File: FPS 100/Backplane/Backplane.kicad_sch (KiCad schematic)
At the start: 27 parts

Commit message: 2026/1/7
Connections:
- net FAOVFL* is gone; now on net FAOVF*: 4401_FA_J1.32
- net FAUNFL* is gone; now on net FAUNF*: 4401_FA_J1.30
- net FAZERO* is gone; now on net FAZRO*: 4422_P1_J3.16
- net SCN is gone; now on net SCIN: 4401_FA_J1.33
- net DE07*: now also 4401_FA_J1.35; no longer 4401_FA_J1.37
- net FRCINH*: now reaches 4401_FA_J2.100
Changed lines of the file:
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@@
 		)
 	)
-	(global_label "FAUNFL*"
+	(global_label "FAUNF*"
 		(shape input)
 		(at 99.06 97.79 0)
@@
 		)
 		(property "Intersheetrefs" "${INTERSHEET_REFS}"
-			(at 109.9677 97.79 0)
+			(at 108.9396 97.79 0)
 			(effects
 				(font
@@
 	(global_label "DE07*"
 		(shape input)
-		(at 86.36 107.95 180)
+		(at 86.36 105.41 180)
 		(fields_autoplaced yes)
 		(effects
@@
 		)
 		(property "Intersheetrefs" "${INTERSHEET_REFS}"
-			(at 77.5692 107.95 0)
+			(at 77.5692 105.41 0)
 			(effects
 				(font
@@
 		)
 	)
-	(global_label "FAZERO*"
+	(global_label "FAZRO*"
 		(shape input)
 		(at 643.89 80.01 0)
@@
 		)
 		(property "Intersheetrefs" "${INTERSHEET_REFS}"
-			(at 654.979 80.01 0)
+			(at 653.83 80.01 0)
 			(effects
 				(font
@@
 		)
 	)
-	(global_label "FAOVFL*"
+	(global_label "FAOVF*"
 		(shape input)
 		(at 99.06 100.33 0)
@@
 		)
 		(property "Intersheetrefs" "${INTERSHEET_REFS}"
-			(at 109.7258 100.33 0)
+			(at 108.6977 100.33 0)
 			(effects
 				(font
@@
 		)
 	)
+	(global_label "FRCINH*"
+		(shape input)
+		(at 99.06 346.71 0)
+		(fields_autoplaced yes)
+		(effects
+			(font
+				(size 1.27 1.27)
+			)
+			(justify left)
+		)
+		(property "Intersheetrefs" "${INTERSHEET_REFS}"
+			(at 109.9072 346.71 0)
+			(effects
+				(font
+					(size 1.27 1.27)
+				)
+				(justify left)
+				(hide yes)
+			)
+		)
+	)
 	(global_label "Y2A1"
 		(shape input)
@@
 		)
 	)
-	(global_label "SCN"
+	(global_label "SCIN"
 		(shape input)
 		(at 86.36 102.87 180)
@@
 		)
 		(property "Intersheetrefs" "${INTERSHEET_REFS}"
-			(at 79.5648 102.87 0)
+			(at 78.96 102.87 0)
 			(effects
 				(font

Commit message: 2026/1/7
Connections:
- net !WRTR is gone; now on net !WRTR*: 4408_P3_J1.9
- net 375LD* is gone; now on net 376LD*: 4422_P1_J3.101
- net B2ID is gone; now on net B2IO: 4421_PDP_IF_J1.42
- net IHRSET* is gone; now on net !HRSET*: 4408_P3_J1.25
- net DPMBS23*: now also 4402_DPL_J2.56
- net DPMBS24*: no longer 4402_DPL_J2.56
- net !HRSET*: now reaches 4421_PDP_IF_J1.52
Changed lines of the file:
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@@
 		)
 	)
-	(global_label "IHRSET*"
+	(global_label "!HRSET*"
 		(shape input)
 		(at 707.39 92.71 180)
@@
 		)
 	)
-	(global_label "B2ID"
+	(global_label "B2IO"
 		(shape input)
 		(at 990.6 113.03 0)
@@
 		)
 		(property "Intersheetrefs" "${INTERSHEET_REFS}"
-			(at 997.9395 113.03 0)
+			(at 998 113.03 0)
 			(effects
 				(font
@@
 		)
 	)
+	(global_label "!HRSET*"
+		(shape input)
+		(at 990.6 125.73 0)
+		(fields_autoplaced yes)
+		(effects
+			(font
+				(size 1.27 1.27)
+			)
+			(justify left)
+		)
+		(property "Intersheetrefs" "${INTERSHEET_REFS}"
+			(at 1001.0842 125.73 0)
+			(effects
+				(font
+					(size 1.27 1.27)
+				)
+				(justify left)
+				(hide yes)
+			)
+		)
+	)
 	(global_label "BUSBGIN"
 		(shape input)
@@
 		)
 	)
-	(global_label "375LD*"
+	(global_label "376LD*"
 		(shape input)
 		(at 631.19 189.23 180)
@@
 		)
 	)
-	(global_label "DPMBS24*"
+	(global_label "DPMBS23*"
 		(shape input)
 		(at 172.72 290.83 0)
@@
 		)
 	)
-	(global_label "!WRTR"
+	(global_label "!WRTR*"
 		(shape input)
 		(at 707.39 72.39 180)
@@
 		)
 		(property "Intersheetrefs" "${INTERSHEET_REFS}"
-			(at 698.841 72.39 0)
+			(at 697.8734 72.39 0)
 			(effects
 				(font

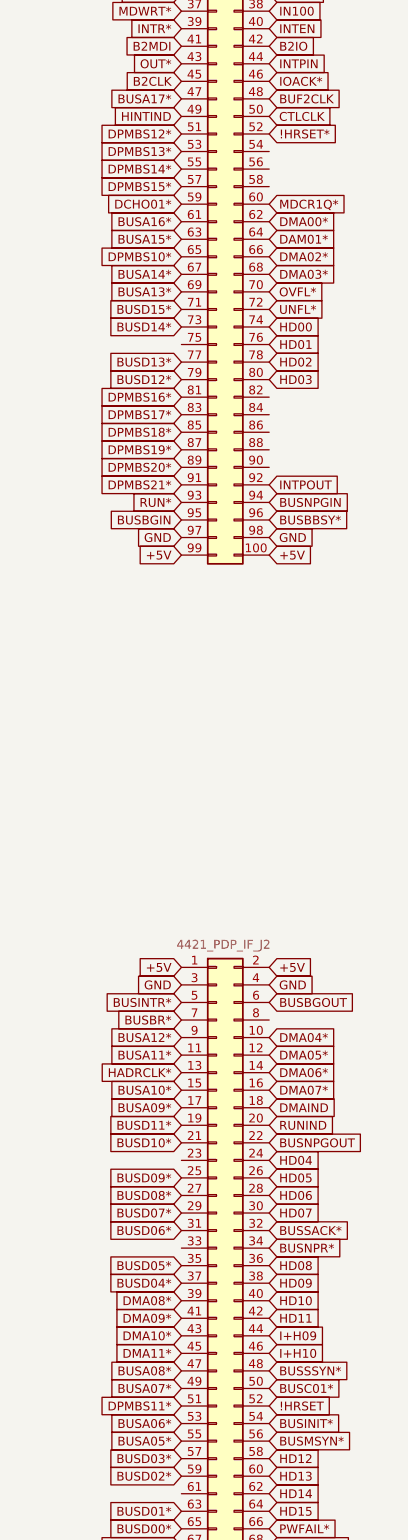
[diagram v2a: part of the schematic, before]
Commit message: 2026/1/8
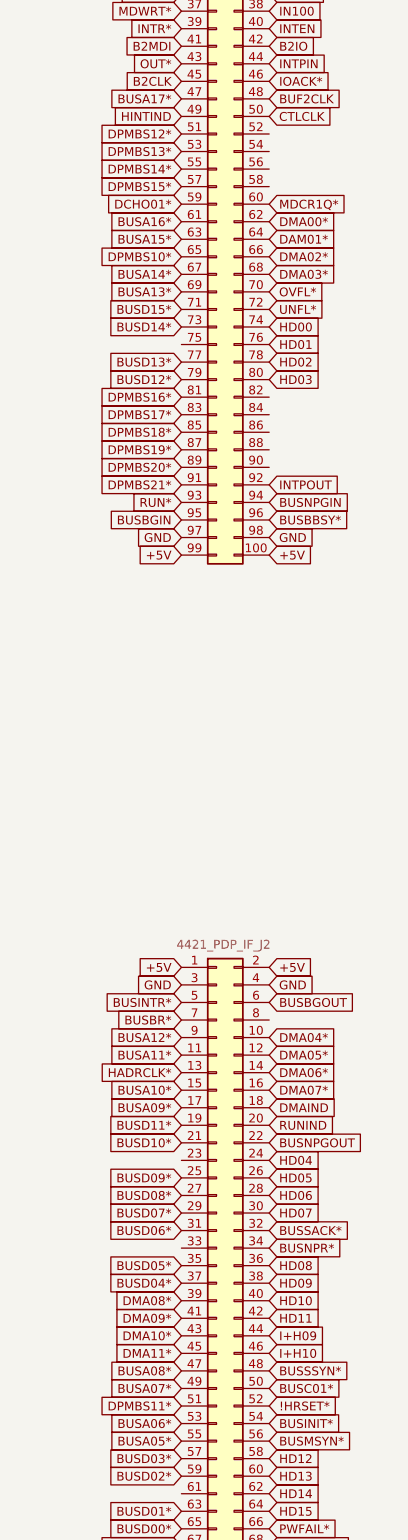
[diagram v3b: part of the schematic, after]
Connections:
- net !HRSET is gone; now on net !HRSET*: 4421_PDP_IF_J2.52
- net !HRSET*: no longer 4421_PDP_IF_J1.52
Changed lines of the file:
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@@
 	(global_label "!HRSET*"
 		(shape input)
-		(at 990.6 125.73 0)
+		(at 990.6 309.88 0)
 		(fields_autoplaced yes)
 		(effects
@@
 		)
 		(property "Intersheetrefs" "${INTERSHEET_REFS}"
-			(at 1001.0842 125.73 0)
+			(at 1001.0842 309.88 0)
 			(effects
 				(font
@@
 			(effects
 				(font
-					(size 1.27 1.27)
-				)
-				(justify left)
-				(hide yes)
-			)
-		)
-	)
-	(global_label "!HRSET"
-		(shape input)
-		(at 990.6 309.88 0)
-		(fields_autoplaced yes)
-		(effects
-			(font
-				(size 1.27 1.27)
-			)
-			(justify left)
-		)
-		(property "Intersheetrefs" "${INTERSHEET_REFS}"
-			(at 1000.1166 309.88 0)
-			(effects
-				(font

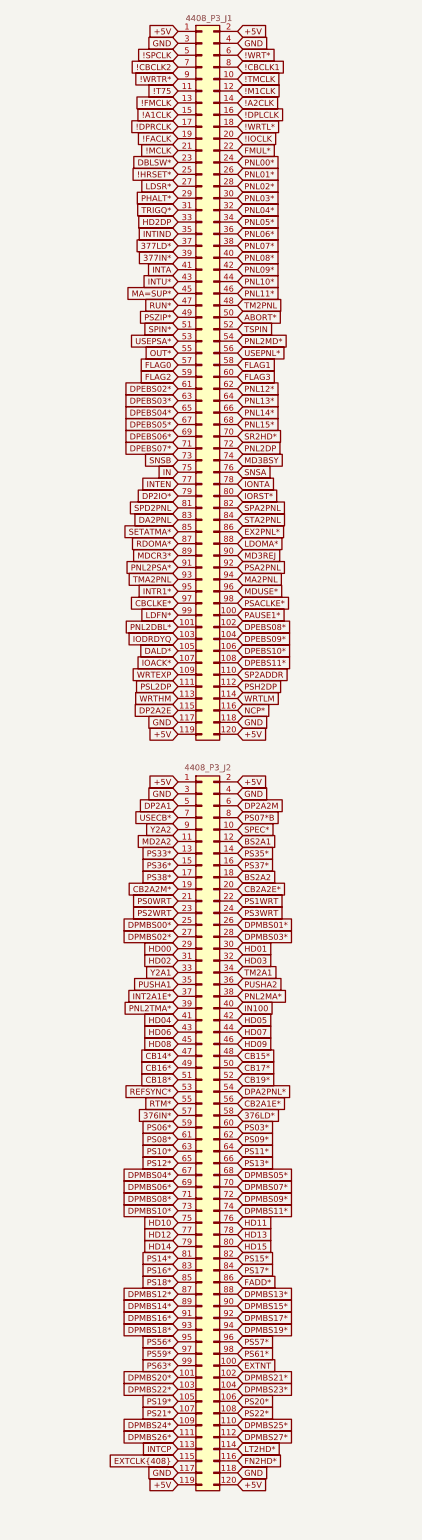
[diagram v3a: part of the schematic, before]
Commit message: 2026/1/8
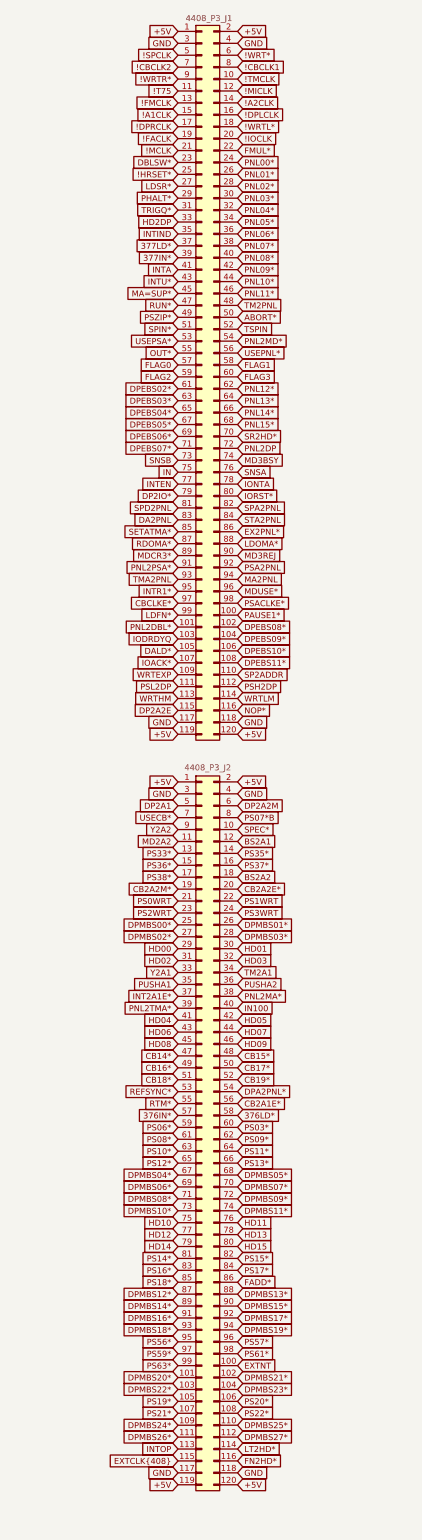
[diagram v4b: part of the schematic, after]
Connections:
- net !M1CLK is gone; now on net !MICLK: 4408_P3_J1.12
- net INTCP is gone; now on net INTOP: 4408_P3_J2.113
- net NCP* is gone; now on net NOP*: 4408_P3_J1.116
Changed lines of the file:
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@@
 		)
 	)
-	(global_label "!M1CLK"
+	(global_label "!MICLK"
 		(shape input)
 		(at 720.09 74.93 0)
@@
 		)
 		(property "Intersheetrefs" "${INTERSHEET_REFS}"
-			(at 729.909 74.93 0)
+			(at 729.3043 74.93 0)
 			(effects
 				(font
@@
 		)
 	)
-	(global_label "NCP*"
+	(global_label "NOP*"
 		(shape input)
 		(at 720.09 207.01 0)
@@
 		)
 		(property "Intersheetrefs" "${INTERSHEET_REFS}"
-			(at 727.9133 207.01 0)
+			(at 727.9738 207.01 0)
 			(effects
 				(font
@@
 		)
 	)
-	(global_label "INTCP"
+	(global_label "INTOP"
 		(shape input)
 		(at 707.39 364.49 180)
@@
 		)
 		(property "Intersheetrefs" "${INTERSHEET_REFS}"
-			(at 698.9619 364.49 0)
+			(at 698.9014 364.49 0)
 			(effects
 				(font

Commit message: 2026/1/8
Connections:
- net DAM01* is gone; now on net DMA01*: 4421_PDP_IF_J1.64
- net MIEBS02* is gone; now on net M1EBS02*: 4425_TM_J1.72
- net MIEBS03* is gone; now on net M1EBS03*: 4425_TM_J1.74
- net MIEBS04* is gone; now on net M1EBS04*: 4425_TM_J1.76
- net MIEBS05* is gone; now on net M1EBS05*: 4425_TM_J1.78
- net MIEBS06* is gone; now on net M1EBS06*: 4425_TM_J1.80
- net MIEBS07* is gone; now on net M1EBS07*: 4425_TM_J1.82
- net MIEBS08* is gone; now on net M1EBS08*: 4425_TM_J1.84
- net MIEBS09* is gone; now on net M1EBS09*: 4425_TM_J1.86
- net MIEBS10* is gone; now on net M1EBS10*: 4425_TM_J1.102
- net MIEBS11* is gone; now on net M1EBS11*: 4425_TM_J1.104
- net MIMBS00* is gone; now on net M1MBS00*: 4425_TM_J1.106
- net MIMBS01* is gone; now on net M1MBS01*: 4425_TM_J1.108
- net MIMBS02* is gone; now on net M1MBS02*: 4425_TM_J1.110
- net MIMBS03* is gone; now on net M1MBS03*: 4425_TM_J1.112
- net MIMBS04* is gone; now on net M1MBS04*: 4425_TM_J1.114
- net MIMBS05* is gone; now on net M1MBS05*: 4425_TM_J1.116
- net MIMBS06* is gone; now on net M1MBS06*: 4425_TM_J2.22
- net MIMBS07* is gone; now on net M1MBS07*: 4425_TM_J2.24
- net MIMBS08* is gone; now on net M1MBS08*: 4425_TM_J2.26
- net MIMBS09* is gone; now on net M1MBS09*: 4425_TM_J2.28
- net MIMBS10* is gone; now on net M1MBS10*: 4425_TM_J2.30
- net MIMBS11* is gone; now on net M1MBS11*: 4425_TM_J2.32
- net MIMBS12* is gone; now on net M1MBS12*: 4425_TM_J2.34
- net MIMBS13* is gone; now on net M1MBS13*: 4425_TM_J2.36
- net MIMBS14* is gone; now on net M1MBS14*: 4425_TM_J2.56
- net MIMBS15* is gone; now on net M1MBS15*: 4425_TM_J2.58
- net MIMBS16* is gone; now on net M1MBS16*: 4425_TM_J2.60
- net MIMBS17* is gone; now on net M1MBS17*: 4425_TM_J2.62
- net MIMBS18* is gone; now on net M1MBS18*: 4425_TM_J2.64
- net MIMBS19* is gone; now on net M1MBS19*: 4425_TM_J2.66
- net MIMBS20* is gone; now on net M1MBS20*: 4425_TM_J2.68
- net MIMBS21* is gone; now on net M1MBS21*: 4425_TM_J2.70
- net MIMBS22* is gone; now on net M1MBS22*: 4425_TM_J2.98
- net MIMBS23* is gone; now on net M1MBS23*: 4425_TM_J2.100
- net MIMBS24* is gone; now on net M1MBS24*: 4425_TM_J2.102
- net MIMBS25* is gone; now on net M1MBS25*: 4425_TM_J2.104
- net MIMBS26* is gone; now on net M1MBS26*: 4425_TM_J2.106
- net MIMBS27* is gone; now on net M1MBS27*: 4425_TM_J2.108
- net PLN00* is gone; now on net PNL00*: 4423_P2_J1.39
- net PLN01* is gone; now on net PNL01*: 4423_P2_J1.40
- net PLN02* is gone; now on net PNL02*: 4423_P2_J1.41
- net PLN03* is gone; now on net PNL03*: 4423_P2_J1.42
- net PLN04* is gone; now on net PNL04*: 4423_P2_J1.43
- net PLN05* is gone; now on net PNL05*: 4423_P2_J1.44
- net PLN06* is gone; now on net PNL06*: 4423_P2_J1.45
- net PLN07* is gone; now on net PNL07*: 4423_P2_J1.46
- net PLN08* is gone; now on net PNL08*: 4423_P2_J1.63
- net PLN09* is gone; now on net PNL09*: 4423_P2_J1.64
- net PLN10* is gone; now on net PNL10*: 4423_P2_J1.65
- net PLN11* is gone; now on net PNL11*: 4423_P2_J1.66
- net PLN12* is gone; now on net PNL12*: 4423_P2_J1.67
- net PLN13* is gone; now on net PNL13*: 4423_P2_J1.68
- net PLN14* is gone; now on net PNL14*: 4423_P2_J1.69
- net PLN15* is gone; now on net PNL15*: 4423_P2_J1.70
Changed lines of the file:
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@@
 		)
 	)
-	(global_label "MIMBS12*"
+	(global_label "M1MBS12*"
 		(shape input)
 		(at 481.33 262.89 0)
@@
 		)
 	)
-	(global_label "MIMBS01*"
+	(global_label "M1MBS01*"
 		(shape input)
 		(at 481.33 196.85 0)
@@
 		)
 	)
-	(global_label "PLN06*"
+	(global_label "PNL06*"
 		(shape input)
 		(at 549.91 118.11 180)
@@
 		)
 	)
-	(global_label "MIMBS09*"
+	(global_label "M1MBS09*"
 		(shape input)
 		(at 481.33 255.27 0)
@@
 		)
 	)
-	(global_label "PLN12*"
+	(global_label "PNL12*"
 		(shape input)
 		(at 549.91 146.05 180)
@@
 		)
 	)
-	(global_label "MIEBS07*"
+	(global_label "M1EBS07*"
 		(shape input)
 		(at 481.33 163.83 0)
@@
 		)
 	)
-	(global_label "MIMBS24*"
+	(global_label "M1MBS24*"
 		(shape input)
 		(at 481.33 349.25 0)
@@
 		)
 	)
-	(global_label "PLN00*"
+	(global_label "PNL00*"
 		(shape input)
 		(at 549.91 110.49 180)
@@
 		)
 	)
-	(global_label "DAM01*"
+	(global_label "DMA01*"
 		(shape input)
 		(at 990.6 140.97 0)
@@
 		)
 	)
-	(global_label "PLN04*"
+	(global_label "PNL04*"
 		(shape input)
 		(at 549.91 115.57 180)
@@
 		)
 	)
-	(global_label "MIMBS08*"
+	(global_label "M1MBS08*"
 		(shape input)
 		(at 481.33 252.73 0)
@@
 		)
 	)
-	(global_label "MIMBS21*"
+	(global_label "M1MBS21*"
 		(shape input)
 		(at 481.33 308.61 0)
@@
 		)
 	)
-	(global_label "MIEBS11*"
+	(global_label "M1EBS11*"
 		(shape input)
 		(at 481.33 191.77 0)
@@
 		)
 	)
-	(global_label "MIEBS06*"
+	(global_label "M1EBS06*"
 		(shape input)
 		(at 481.33 161.29 0)
@@
 		)
 	)
-	(global_label "PLN01*"
+	(global_label "PNL01*"
 		(shape input)
 		(at 562.61 110.49 0)
@@
 		)
 	)
-	(global_label "PLN03*"
+	(global_label "PNL03*"
 		(shape input)
 		(at 562.61 113.03 0)
@@
 		)
 	)
-	(global_label "MIMBS06*"
+	(global_label "M1MBS06*"
 		(shape input)
 		(at 481.33 247.65 0)
@@
 		)
 	)
-	(global_label "MIMBS23*"
+	(global_label "M1MBS23*"
 		(shape input)
 		(at 481.33 346.71 0)
@@
 		)
 	)
-	(global_label "MIMBS03*"
+	(global_label "M1MBS03*"
 		(shape input)
 		(at 481.33 201.93 0)
@@
 		)
 	)
-	(global_label "MIEBS02*"
+	(global_label "M1EBS02*"
 		(shape input)
 		(at 481.33 151.13 0)
@@
 		)
 	)
-	(global_label "MIMBS11*"
+	(global_label "M1MBS11*"
 		(shape input)
 		(at 481.33 260.35 0)
@@
 		)
 	)
-	(global_label "PLN05*"
+	(global_label "PNL05*"
 		(shape input)
 		(at 562.61 115.57 0)
@@
 		)
 	)
-	(global_label "PLN11*"
+	(global_label "PNL11*"
 		(shape input)
 		(at 562.61 143.51 0)
@@
 		)
 	)
-	(global_label "MIEBS08*"
+	(global_label "M1EBS08*"
 		(shape input)
 		(at 481.33 166.37 0)
@@
 		)
 	)
-	(global_label "MIMBS14*"
+	(global_label "M1MBS14*"
 		(shape input)
 		(at 481.33 290.83 0)
@@
 		)
 	)
-	(global_label "MIMBS19*"
+	(global_label "M1MBS19*"
 		(shape input)
 		(at 481.33 303.53 0)
@@
 		)
 	)
-	(global_label "MIEBS05*"
+	(global_label "M1EBS05*"
 		(shape input)
 		(at 481.33 158.75 0)
@@
 		)
 	)
-	(global_label "MIMBS27*"
+	(global_label "M1MBS27*"
 		(shape input)
 		(at 481.33 356.87 0)
@@
 		)
 	)
-	(global_label "MIMBS22*"
+	(global_label "M1MBS22*"
 		(shape input)
 		(at 481.33 344.17 0)
@@
 		)
 	)
-	(global_label "MIMBS16*"
+	(global_label "M1MBS16*"
 		(shape input)
 		(at 481.33 295.91 0)
@@
 		)
 	)
-	(global_label "MIMBS26*"
+	(global_label "M1MBS26*"
 		(shape input)
 		(at 481.33 354.33 0)
@@
 		)
 	)
-	(global_label "MIMBS02*"
+	(global_label "M1MBS02*"
 		(shape input)
 		(at 481.33 199.39 0)
@@
 		)
 	)
-	(global_label "PLN13*"
+	(global_label "PNL13*"
 		(shape input)
 		(at 562.61 146.05 0)
@@
 		)
 	)
-	(global_label "MIMBS05*"
+	(global_label "M1MBS05*"
 		(shape input)
 		(at 481.33 207.01 0)
@@
 		)
 	)
-	(global_label "MIMBS18*"
+	(global_label "M1MBS18*"
 		(shape input)
 		(at 481.33 300.99 0)
@@
 		)
 	)
-	(global_label "MIMBS00*"
+	(global_label "M1MBS00*"
 		(shape input)
 		(at 481.33 194.31 0)
@@
 		)
 	)
-	(global_label "MIMBS15*"
+	(global_label "M1MBS15*"
 		(shape input)
 		(at 481.33 293.37 0)
@@
 		)
 	)
-	(global_label "PLN08*"
+	(global_label "PNL08*"
 		(shape input)
 		(at 549.91 140.97 180)
@@
 		)
 	)
-	(global_label "PLN02*"
+	(global_label "PNL02*"
 		(shape input)
 		(at 549.91 113.03 180)
@@
 		)
 	)
-	(global_label "PLN14*"
+	(global_label "PNL14*"
 		(shape input)
 		(at 549.91 148.59 180)
@@
 		)
 	)
-	(global_label "PLN15*"
+	(global_label "PNL15*"
 		(shape input)
 		(at 562.61 148.59 0)
@@
 		)
 	)
-	(global_label "PLN07*"
+	(global_label "PNL07*"
 		(shape input)
 		(at 562.61 118.11 0)
@@
 		)
 	)
-	(global_label "MIMBS07*"
+	(global_label "M1MBS07*"
 		(shape input)
 		(at 481.33 250.19 0)
@@
 		)
 	)
-	(global_label "MIMBS20*"
+	(global_label "M1MBS20*"
 		(shape input)
 		(at 481.33 306.07 0)
@@
 		)
 	)
-	(global_label "MIEBS03*"
+	(global_label "M1EBS03*"
 		(shape input)
 		(at 481.33 153.67 0)
@@
 		)
 	)
-	(global_label "MIMBS04*"
+	(global_label "M1MBS04*"
 		(shape input)
 		(at 481.33 204.47 0)
@@
 		)
 	)
-	(global_label "PLN10*"
+	(global_label "PNL10*"
 		(shape input)
 		(at 549.91 143.51 180)
@@
 		)
 	)
-	(global_label "MIMBS13*"
+	(global_label "M1MBS13*"
 		(shape input)
 		(at 481.33 265.43 0)
@@
 		)
 	)
-	(global_label "MIMBS25*"
+	(global_label "M1MBS25*"
 		(shape input)
 		(at 481.33 351.79 0)
@@
 		)
 	)
-	(global_label "MIMBS17*"
+	(global_label "M1MBS17*"
 		(shape input)
 		(at 481.33 298.45 0)
@@
 		)
 	)
-	(global_label "MIMBS10*"
+	(global_label "M1MBS10*"
 		(shape input)
 		(at 481.33 257.81 0)
@@
 		)
 	)
-	(global_label "PLN09*"
+	(global_label "PNL09*"
 		(shape input)
 		(at 562.61 140.97 0)
@@
 		)
 	)
-	(global_label "MIEBS04*"
+	(global_label "M1EBS04*"
 		(shape input)
 		(at 481.33 156.21 0)
@@
 		)
 	)
-	(global_label "MIEBS10*"
+	(global_label "M1EBS10*"
 		(shape input)
 		(at 481.33 189.23 0)
@@
 		)
 	)
-	(global_label "MIEBS09*"
+	(global_label "M1EBS09*"
 		(shape input)
 		(at 481.33 168.91 0)
